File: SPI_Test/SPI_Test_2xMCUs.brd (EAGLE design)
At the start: 120 x 145 mm, 82 parts, among them J1 10-pos, J13 4-pos, J25 10-pos, J4 10-pos, U1 RENESAS_R7FS5D37A3A01CFM#AA0P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, U13 RENESAS_R7FS5D37A3A01CFM#AA0P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, U2 S7G2LQFP176, X14 32.768KHz, X2 32.768KHz, X3 32.768KHz, X4 24MHz, Y1 XTAL_12MHZ_ABM8G-12.000MHZ-B4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, Y12 XTAL_12MHZ_ABM8G-12.000MHZ-B4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

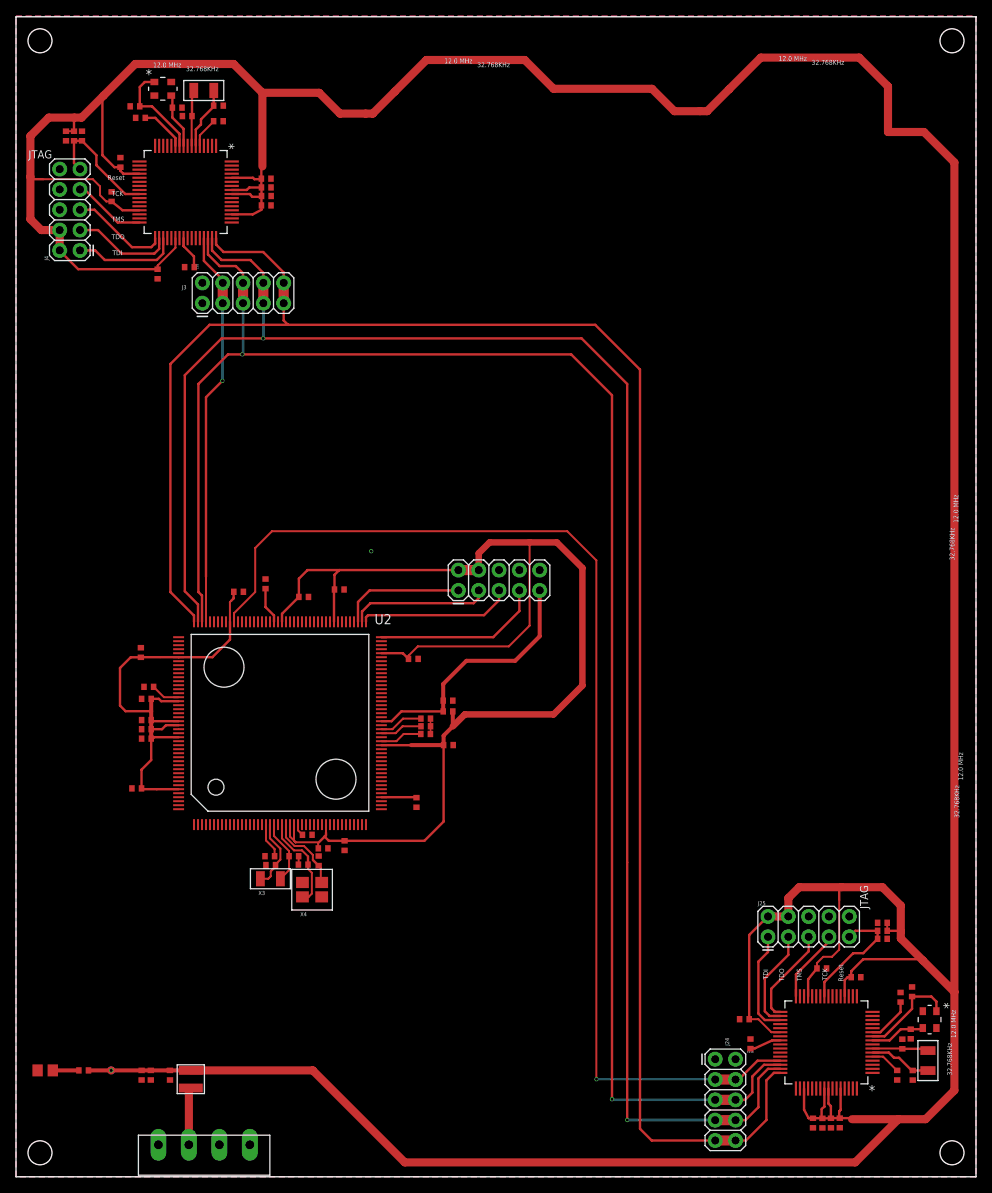
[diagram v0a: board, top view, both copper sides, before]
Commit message: update
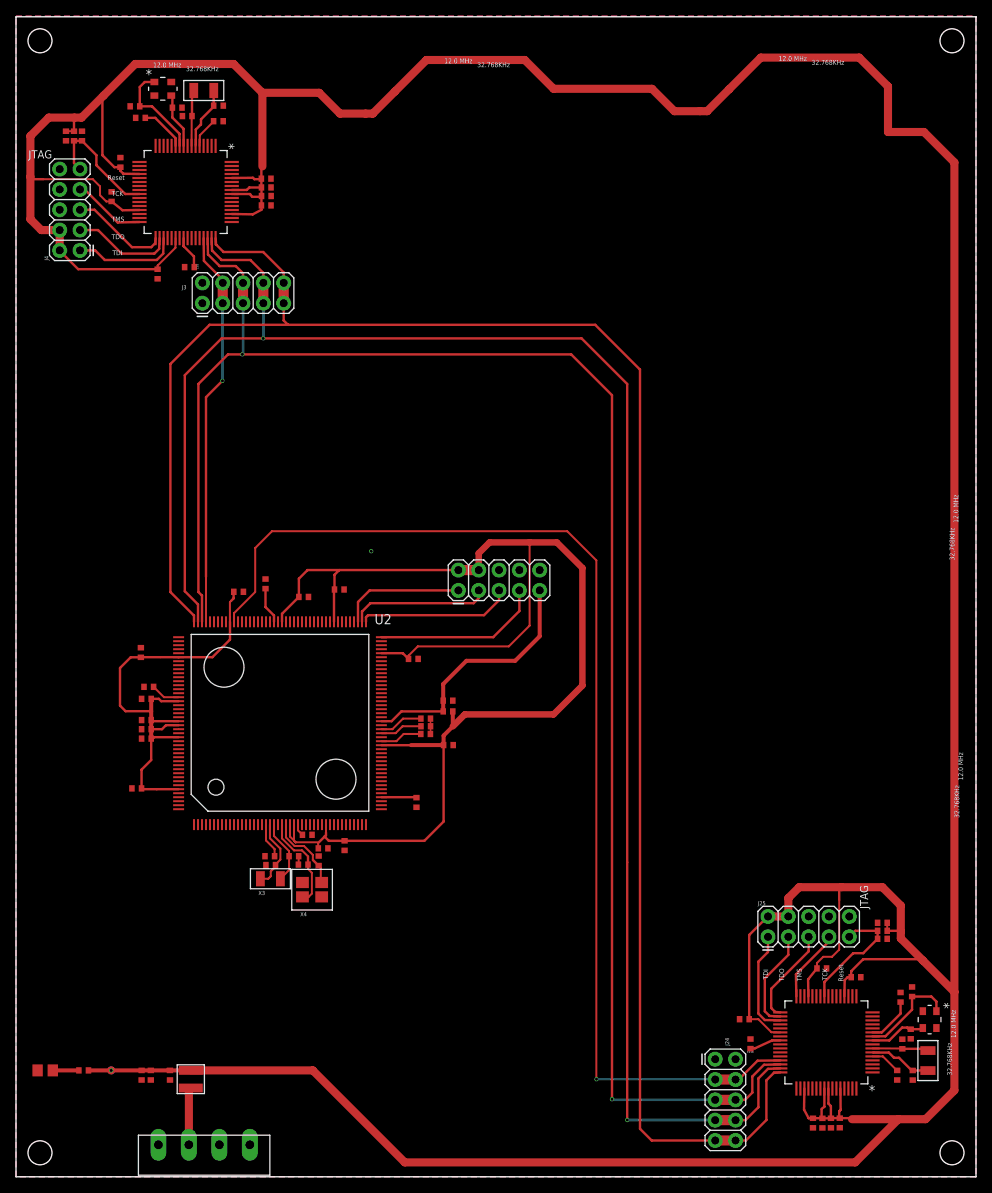
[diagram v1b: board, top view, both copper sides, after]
